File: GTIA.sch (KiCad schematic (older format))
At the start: 76 parts, among them J102 pin, J103 pin, J104 pin, J105 pin, J2 Video, Q1 2N3904, Q2 2N3904, Q3 2N3904, Q6 2N3904, U17 GTIA, U18 74LS08, U20 4050, U21 74LS74, Y2 4,43 MHz

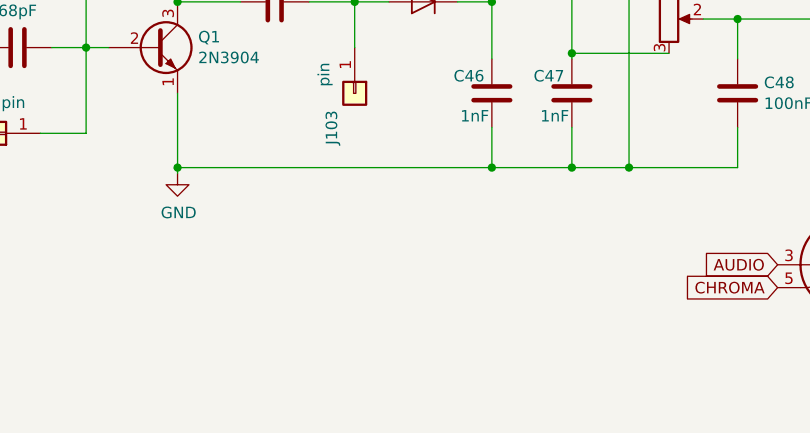
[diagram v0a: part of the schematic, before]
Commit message: Trackimg
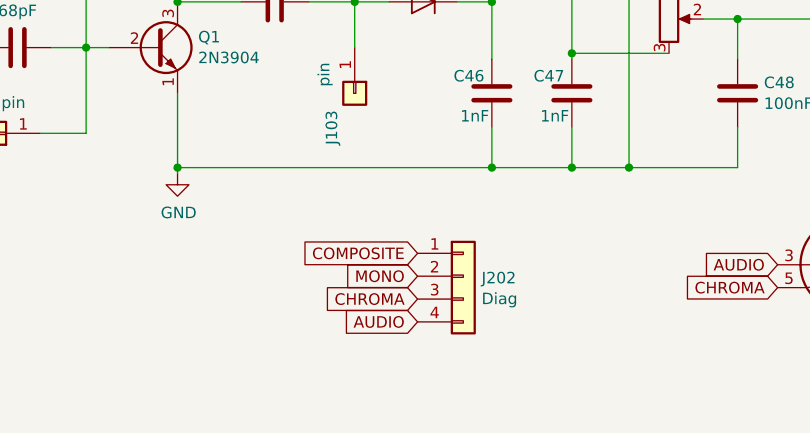
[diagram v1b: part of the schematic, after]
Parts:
- added J202: Diag, Connector_PinHeader_2.54mm:PinHeader_1x04_P2.54mm_Vertical, symbol Connector_Generic:Conn_01x04
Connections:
- net AUDIO: now also J202.4 (Pin_4)
- net CHROMA: now also J202.3 (Pin_3)
- net COMPOSITE: now also J202.1 (Pin_1)
- net MONO: now also J202.2 (Pin_2)
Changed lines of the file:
@@
 	6150 7350 6150 7125
 Connection ~ 6150 7125
+Text GLabel 2650 7200 0    50   Input ~ 0
+MONO
+Text GLabel 2650 7100 0    50   Input ~ 0
+COMPOSITE
+Text GLabel 2650 7300 0    50   Input ~ 0
+CHROMA
+Text GLabel 2650 7400 0    50   Input ~ 0
+AUDIO
+$Comp
+L Connector_Generic:Conn_01x04 J202
+U 1 1 6046696D
+P 2850 7200
+F 0 "J202" H 2930 7192 50  0000 L CNN
+F 1 "Diag" H 2930 7101 50  0000 L CNN
+F 2 "Connector_PinHeader_2.54mm:PinHeader_1x04_P2.54mm_Vertical" H 2850 7200 50  0001 C CNN
+F 3 "~" H 2850 7200 50  0001 C CNN
+	1    2850 7200
+	1    0    0    -1
+$EndComp
 $EndSCHEMATC
